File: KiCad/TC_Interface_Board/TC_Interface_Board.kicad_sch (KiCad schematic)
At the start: 30 parts, among them J1 Conn_01x05, J1_24V1 JST_VH_01x04, J1_CN1 JST_VH_01x03, J2 Conn_01x05, J2_CN1 JST_VH_01x02, J3 Conn_01x05, J3_CN1 JST_VH_01x02, J4 Conn_01x05, J5 Conn_01x05, J6 Conn_01x05, J7 Conn_01x05, J8 Conn_01x05, Q1 DTC143E, Q2 DTC143E, U1 MC34063AP

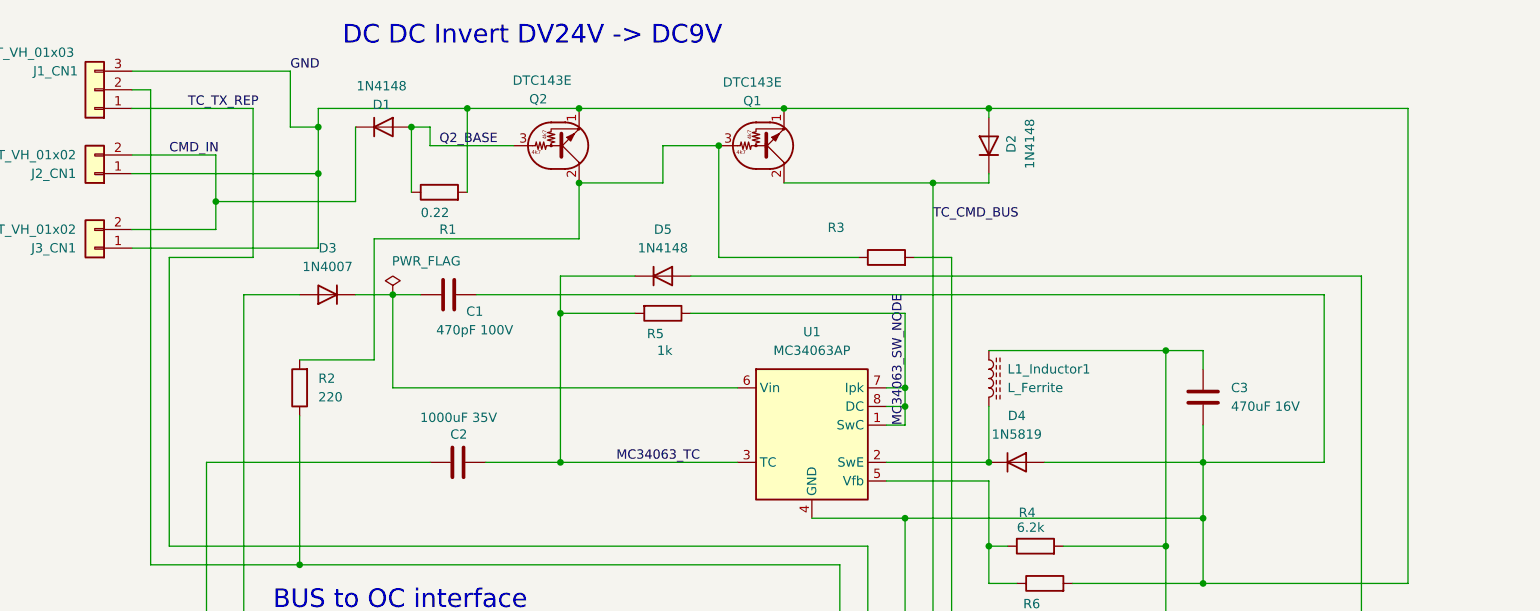
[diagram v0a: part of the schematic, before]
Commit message: UPDATE
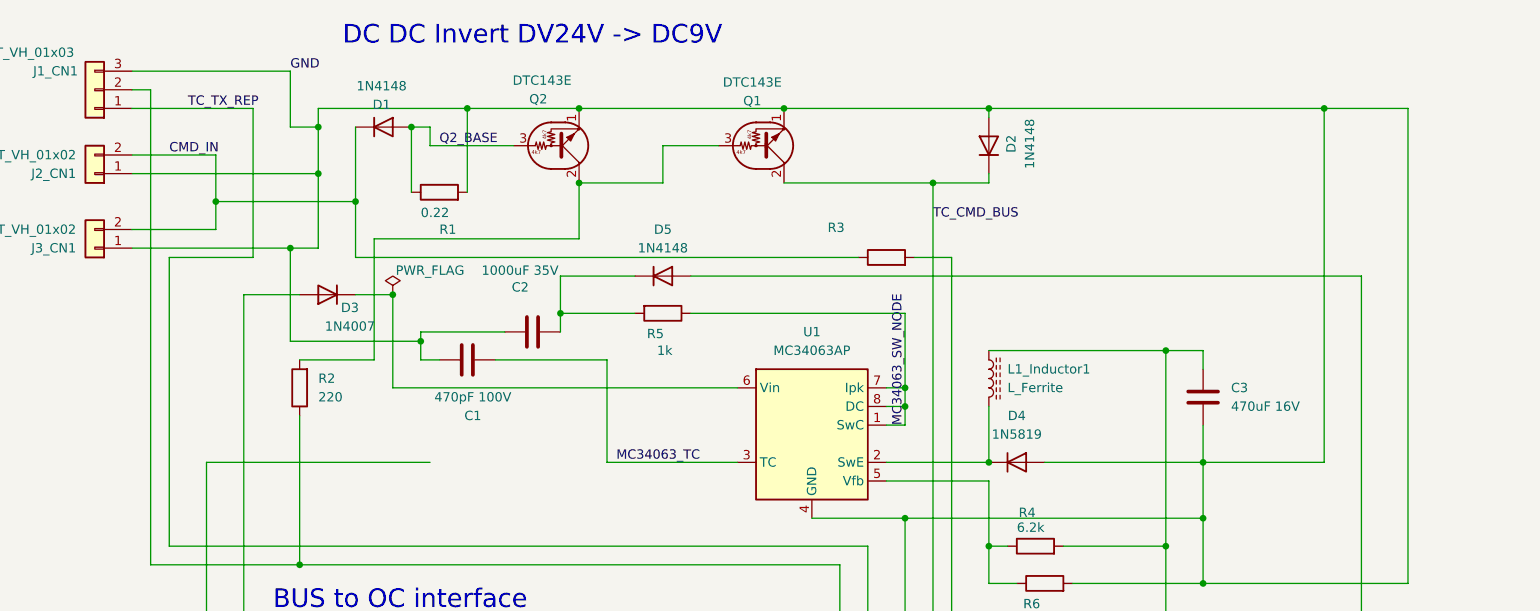
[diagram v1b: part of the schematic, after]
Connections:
- net CMD_IN: now also R3.1
- net MC34063_TC: now also C1.1; no longer C2.1, D5.1 (K), R5.2
- net at D3.1 (K), U1.6 (Vin): no longer C1.1
- net at Q1.3 (B), Q2.2 (C), R2.2: no longer R3.1
- new net: C2.1, D5.1 (K), R5.2
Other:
- moved on the sheet: C1, C2
